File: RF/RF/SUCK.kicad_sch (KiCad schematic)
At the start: 1 part, among them J801 ESQ-110-13-G-D

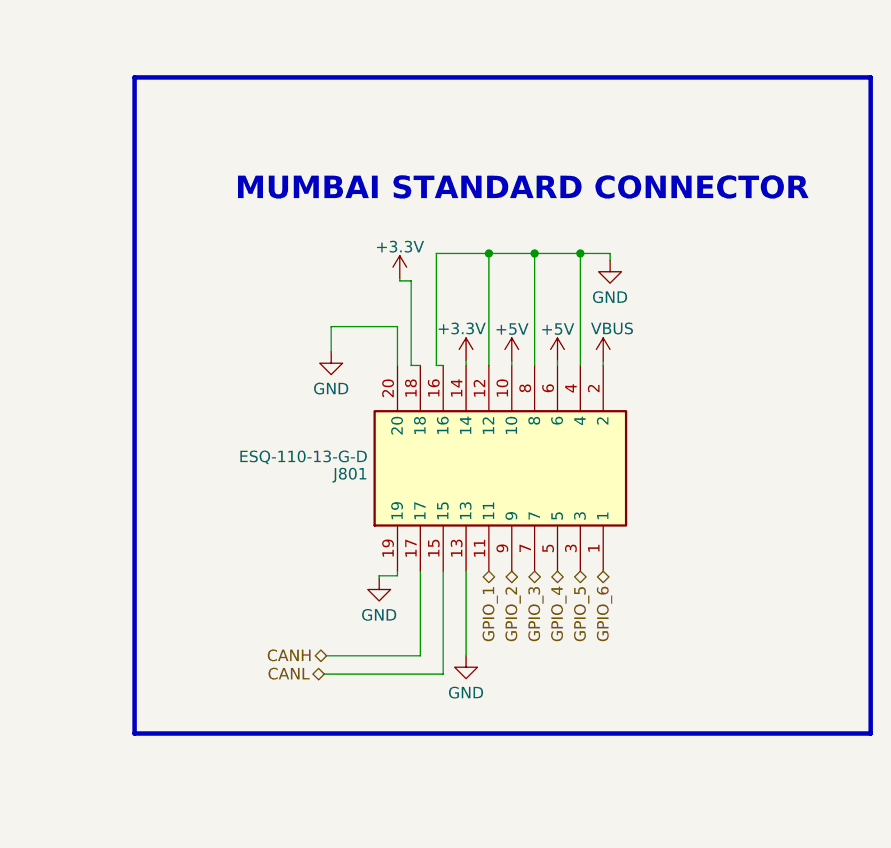
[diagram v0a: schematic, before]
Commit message: layout rev 1.0
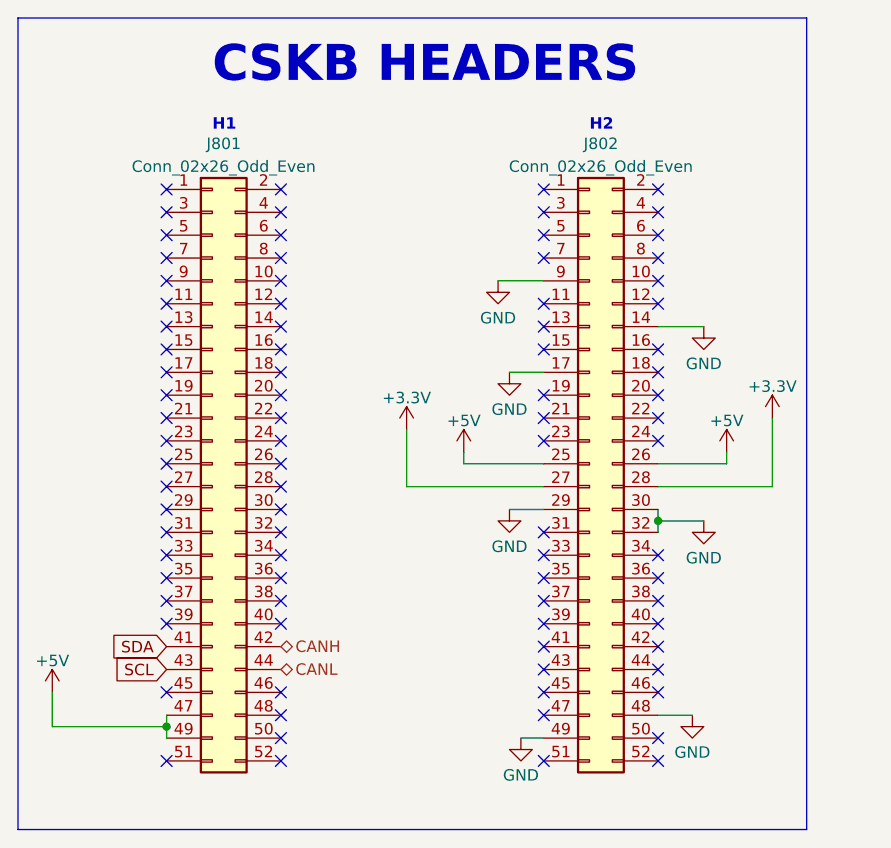
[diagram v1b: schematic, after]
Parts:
- removed J801: ESQ-110-13-G-D, SamacSys_Parts:ESQ-110-Y-X-D, symbol SamacSys_Parts:ESQ-110-13-G-D
- added J801, J802: Conn_02x26_Odd_Even, Connector_PinSocket_2.54mm:PinSocket_2x26_P2.54mm_Vertical, symbol Connector_Generic:Conn_02x26_Odd_Even
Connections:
- net +3.3V: now also J802.27 (Pin_27), J802.28 (Pin_28)
- net +5V: now also J801.47 (Pin_47), J801.49 (Pin_49), J802.25 (Pin_25), J802.26 (Pin_26)
- net CANH: now also J801.42 (Pin_42)
- net CANL: now also J801.44 (Pin_44)
- net GND: now also J802.14 (Pin_14), J802.17 (Pin_17), J802.29 (Pin_29), J802.30 (Pin_30), J802.32 (Pin_32), J802.48 (Pin_48), J802.49 (Pin_49), J802.9 (Pin_9)
- new net SCL: J801.43 (Pin_43)
- new net SDA: J801.41 (Pin_41)
- no-connect marks 0 -> 86
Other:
- note added: "CSKB HEADERS"
- note added: "H1"
- note added: "H2"
- note removed: "MUMBAI STANDARD CONNECTOR"
